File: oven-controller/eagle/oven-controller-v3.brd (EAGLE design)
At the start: 74.3 x 45.4 mm, 48 parts, among them Q1 FDV305N, Q2 FDV305N, Q3 FDV305N, Q4 FDV305N, U1 ARDUINO_SHIELDLONGPADS, U2 MAX31855, U3 MAX31855, U4 MAX31855, U5 MAX31855, U6 MAX31855

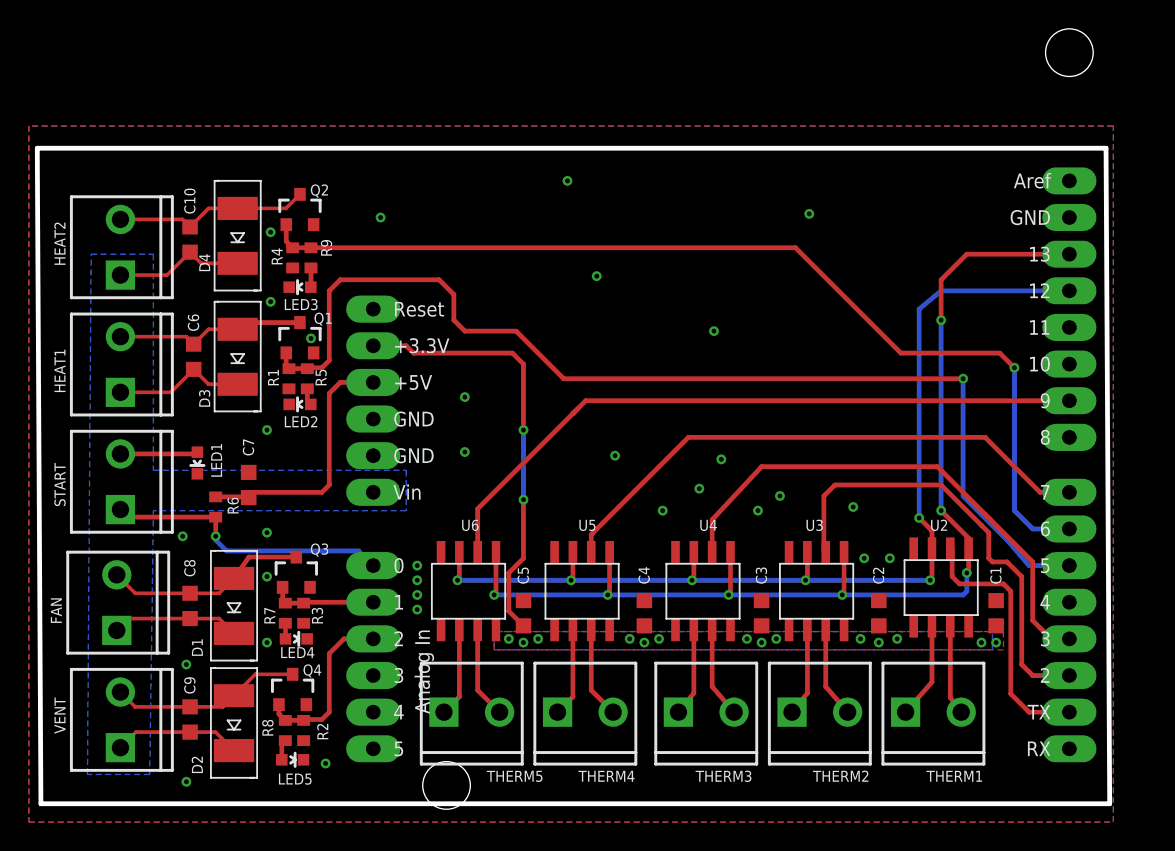
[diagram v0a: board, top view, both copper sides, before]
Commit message: Lots of fixes. Reviewed. Passes ERC, DRC, rats. Ship it.
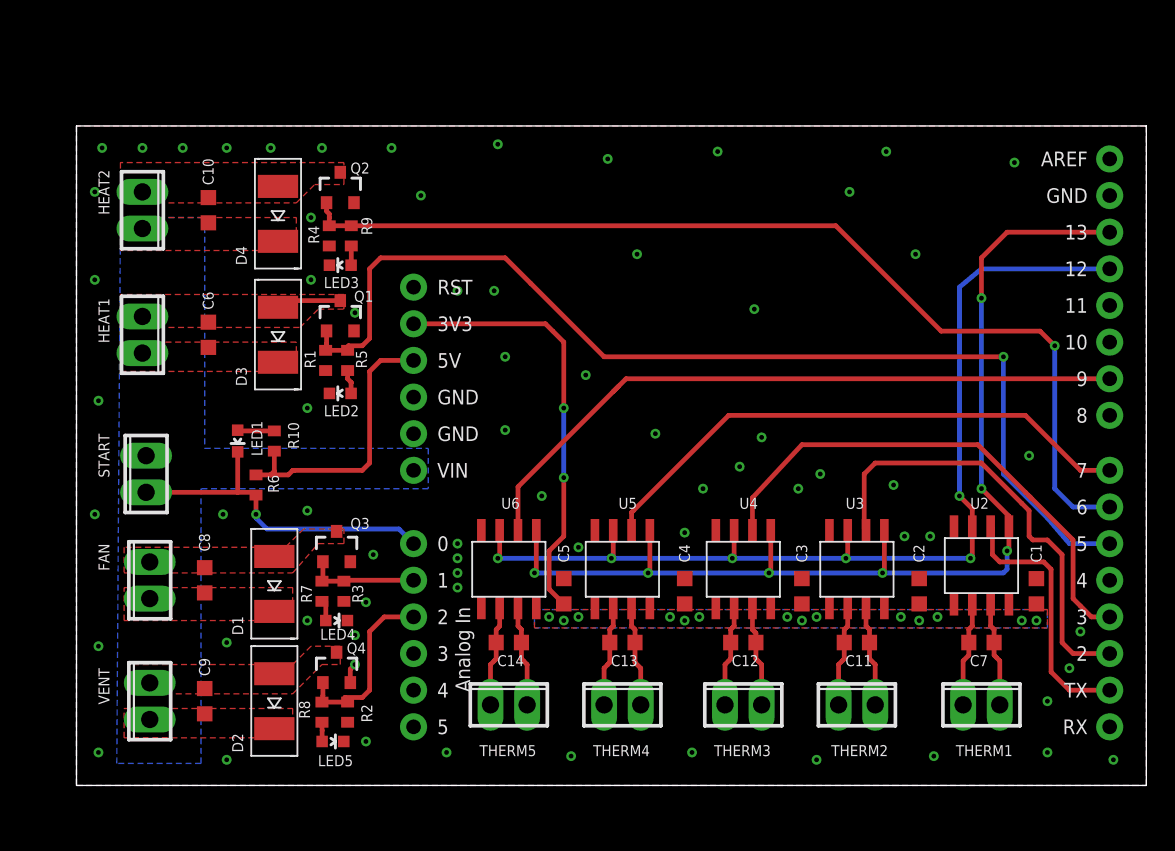
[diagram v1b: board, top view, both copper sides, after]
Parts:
- added C11, C12, C13, C14: 10n, rcl_custom:C0603K
- added R10: 1k, rcl_custom:0603-C-NOSILK
- C10, C6, C8, C9: value 100n -> 100n 100V
- C7: value 100n -> 10n
- FAN: value HDR4 -> (none); device SparkFun-Connectors:SCREWTERMINAL-3.5MM-2_LOCK -> con-phoenix-254:2POL254
- HEAT1: value HDR2 -> (none); device SparkFun-Connectors:SCREWTERMINAL-3.5MM-2_LOCK -> con-phoenix-254:2POL254
- HEAT2: value HDR3 -> (none); device SparkFun-Connectors:SCREWTERMINAL-3.5MM-2_LOCK -> con-phoenix-254:2POL254
- R5, R7, R8, R9: value 330 -> 1k
- R6: value 330 -> 10k
- START: value HDR1 -> (none); device SparkFun-Connectors:SCREWTERMINAL-3.5MM-2_LOCK -> con-phoenix-254:2POL254
- THERM1, THERM2, THERM3, THERM4, THERM5: device SparkFun-Connectors:SCREWTERMINAL-3.5MM-2_LOCK -> con-phoenix-254:2POL254
- U1: value ARDUINO_SHIELDLONGPADS -> ARDUINO_SHIELDNOHOLES; device SparkFun-Boards:DUEMILANOVE_SHIELD_LONGPADS -> SparkFun-Boards:DUEMILANOVE_SHIELD_NOHOLES
- VENT: value HDR5 -> (none); device SparkFun-Connectors:SCREWTERMINAL-3.5MM-2_LOCK -> con-phoenix-254:2POL254
- moved C7 52.0 mm to (62.7, 9.91), turned to 0 degrees
- moved THERM1 5.11 mm to (62.7, 5.59)
- moved HEAT2 4.58 mm to (4.57, 39.9), turned to 270 degrees
- moved THERM3 4.35 mm to (46.2, 5.59)
- moved THERM5 4.35 mm to (30.0, 5.59)
- moved THERM2 4.35 mm to (54.1, 5.59)
- moved THERM4 4.35 mm to (37.8, 5.59)
- moved HEAT1 4.10 mm to (4.57, 31.2), turned to 270 degrees
- moved FAN 4.02 mm to (5.08, 14.2)
- moved VENT 3.66 mm to (5.08, 5.84)
- moved Q4 3.41 mm to (18.0, 8.13)
- moved Q3 3.31 mm to (18.0, 16.5)
- moved R2 3.30 mm to (18.8, 5.08)
- moved U1 3.18 mm to (74.2, 58.7)
- moved U4 3.18 mm to (46.2, 15.0)
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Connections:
- net CS_FAN renamed FAN_EN
- net CS_HEAT1 renamed HEAT1_EN
- net CS_HEAT2 renamed HEAT2_EN
- net CS_VENT renamed VENT_EN
- net THERM_CS1 renamed THERM_!CS1
- net THERM_CS2 renamed THERM_!CS2
- net THERM_CS3 renamed THERM_!CS3
- net THERM_CS4 renamed THERM_!CS4
- net THERM_CS5 renamed THERM_!CS5
- removed net N$11: THERM2.2, U3.3
- removed net N$14: THERM4.1, U5.2
- removed net N$16: THERM5.1, U6.2
- removed net START: R6.1, START.1, U1.A0
- new net !START: LED1.C, R6.1, START.1, U1.A0
- new net N$1: LED1.A, R10.1
- new net N$10: C12.1, THERM3.1, U4.2
- new net N$20: C12.2, THERM3.2, U4.3
- net 12V: now also HEAT1.2, HEAT2.2; no longer HEAT1.1, HEAT2.1
- net 5V: now also R10.2; no longer C7.1
- net GND: now also START.2; no longer C7.2, LED1.C
- net N$12: now also C11.1, THERM2.1, U3.2; no longer THERM3.1, U4.2
- net N$13: now also C11.2, THERM2.2, U3.3; no longer THERM3.2, U4.3
- net N$15: now also C14.2, THERM5.2, U6.3; no longer THERM4.2, U5.3
- net N$17: now also C14.1, THERM5.1, U6.2; no longer THERM5.2, U6.3
- net N$2: now also C7.1, THERM1.1, U2.2; no longer LED1.A, START.2
- net N$21: now also HEAT2.1; no longer HEAT2.2
- net N$4: now also HEAT1.1; no longer HEAT1.2
- net N$5: now also C7.2, THERM1.2, U2.3; no longer THERM1.1, U2.2
- net N$6: now also C13.1, THERM4.1, U5.2; no longer THERM1.2, U2.3
- net N$8: now also C13.2, THERM4.2, U5.3; no longer THERM2.1, U3.2
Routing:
- net 12V: track 36.1 -> 0.00 mm
- net !START: track 0.00 -> 23.8 mm, vias 0 -> 1
- net START: track 20.1 -> 0.00 mm, vias 1 -> 0
- net HDR3: track 14.2 -> 0.00 mm
- net N$21: track 13.6 -> 0.00 mm
- net N$3: track 13.3 -> 0.00 mm
- net N$4: track 13.5 -> 4.76 mm
- net N$10: track 0.00 -> 6.97 mm
- net N$20: track 0.00 -> 6.97 mm
- net N$11: track 6.25 -> 0.00 mm
- net N$16: track 6.13 -> 0.00 mm
- net N$14: track 6.13 -> 0.00 mm
- net N$1: track 0.00 -> 2.56 mm
- net N$2: track 5.38 -> 7.23 mm
- net 5V: track 18.0 -> 19.7 mm
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- added copper zone on layer 1, net 12V
- added copper zone on layer 1, net HDR3
- added copper zone on layer 1, net N$21
- added copper zone on layer 1, net N$3
- added copper zone on layer 1, net N$4
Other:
- board size 74.3 x 45.4 mm -> 74.2 x 45.7 mm
